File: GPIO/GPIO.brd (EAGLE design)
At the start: 35.6 x 29.8 mm, 30 parts

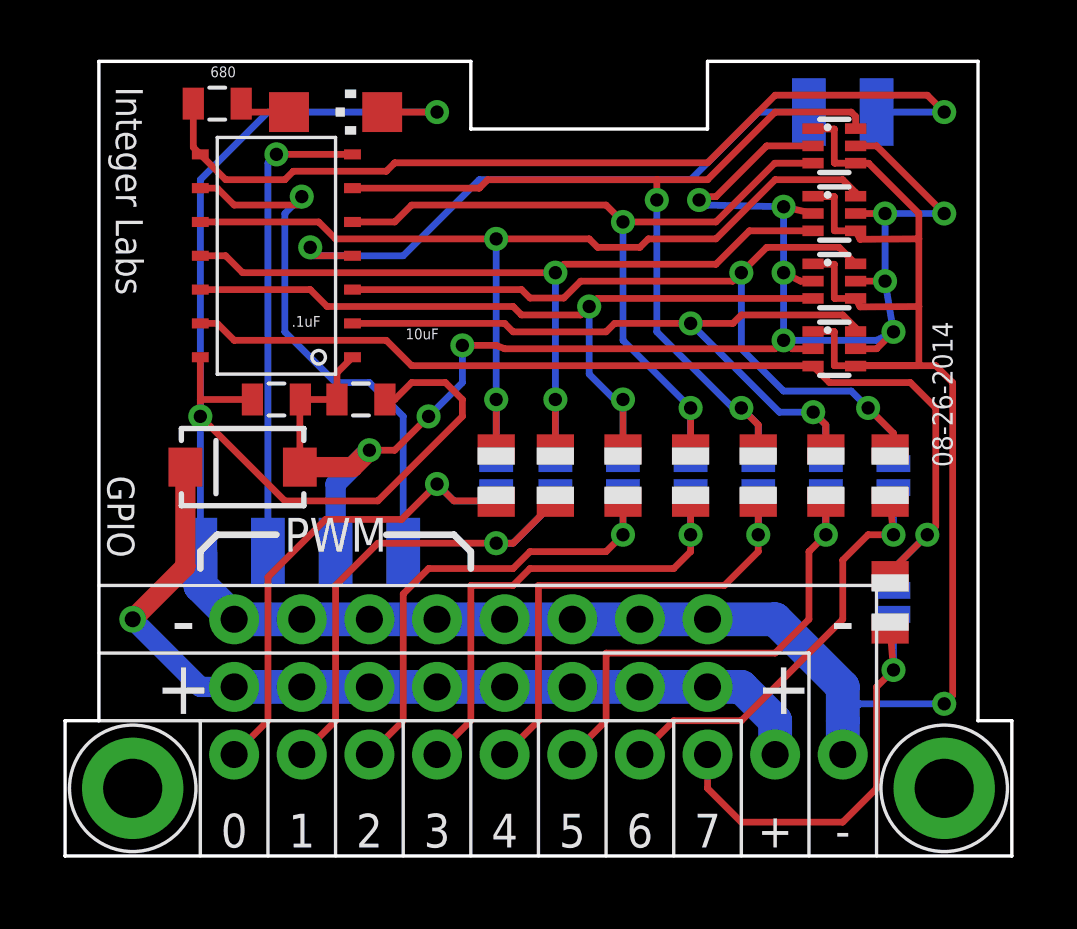
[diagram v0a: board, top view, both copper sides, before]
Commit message: Latest version of schematics and boards
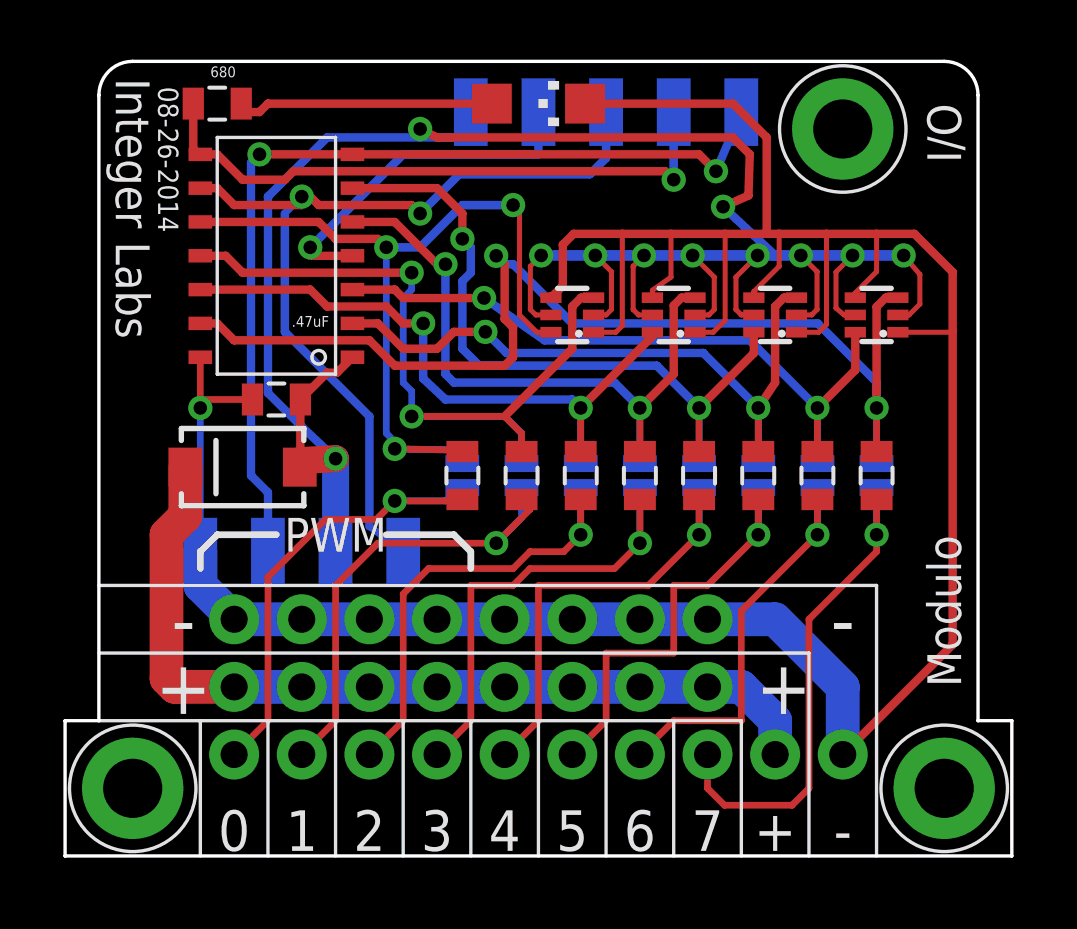
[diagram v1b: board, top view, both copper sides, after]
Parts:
- removed C1: 10uF, SparkFun-Capacitors:0805
- removed D0, D3, D5, D7: BAS70XY, diode:SOT363_PHILIPS
- added D26, D27, D28, D29: BAS70XY, diode:SOT363_PHILIPS
- C2: value .1uF -> .47uF
- R10, R11, R12, R13, R14, R15, R8, R9: value (none) -> 200; device adafruit:R0805 -> SparkFun-Resistors:0805
- moved LED 7.63 mm to (17.8, 28.3)
- moved R7 4.80 mm to (30.5, 14.3)
- moved R8 4.79 mm to (30.5, 14.3)
- moved R4 2.86 mm to (28.3, 14.3)
- moved R9 2.73 mm to (28.3, 14.3)
- moved R10 2.54 mm to (26.0, 14.3)
- moved R6 2.54 mm to (26.0, 14.3)
- moved R0 2.22 mm to (23.8, 14.3)
- moved R11 2.22 mm to (23.8, 14.3)
- moved R1 1.91 mm to (21.6, 14.3)
- moved R12 1.91 mm to (21.6, 14.3)
- moved R13 1.59 mm to (19.4, 14.3)
- moved R5 1.59 mm to (19.4, 14.3)
- moved R14 1.27 mm to (17.1, 14.3)
- moved R15 1.27 mm to (14.9, 14.3)
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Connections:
- net GND: now also D26.1, D26.4, D27.1, D27.4, D28.1, D28.4, D29.1, D29.4, U$4.BUS0; no longer C1.1, D0.1, D0.4, D3.1, D3.4, D5.1, D5.4, D7.1, D7.4, U$4.GND
- net GPIO0: now also D26.6; no longer D3.6
- net GPIO1: now also D26.3; no longer D3.3
- net GPIO2: now also D27.6; no longer D5.3
- net GPIO3: now also D27.3; no longer D0.3
- net GPIO4: now also D28.6; no longer D0.6
- net GPIO5: now also D28.3; no longer D7.6
- net GPIO6: now also D29.6; no longer D5.6
- net GPIO7: now also D29.3; no longer D7.3
- net MISO/LED: now also U$4.PROG3; no longer U$4.MISO
- net RESET: now also U$4.PROG1; no longer U$4.RESET
- net SCL/SCK: now also U$4.BUS3, U$4.PROG2; no longer U$4.SCL
- net SDA/MOSI: now also U$4.BUS1, U$4.PROG4; no longer U$4.SDA
- net VCC: now also D26.2, D26.5, D27.2, D27.5, D28.2, D28.5, D29.2, D29.5, U$4.BUS2, U$4.PROG0; no longer C1.2, D0.2, D0.5, D3.2, D3.5, D5.2, D5.5, D7.2, D7.5, U$4.VCC
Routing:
- net VCC: track 67.7 -> 87.3 mm
- net SDA/MOSI: track 17.9 -> 35.1 mm, vias 1 -> 2
- net SCL/SCK: track 20.6 -> 34.2 mm, vias 1 -> 2
- net GND: track 124.7 -> 112.0 mm, vias 3 -> 1
- net MISO/LED: track 34.5 -> 23.0 mm
- net RESET: track 23.2 -> 13.5 mm
- net N$5: track 1.93 -> 9.68 mm
- net GPIO4: track 34.8 -> 27.1 mm
- net GPIO2: track 32.1 -> 25.2 mm
- net GPIO6: track 33.0 -> 26.3 mm
- net GPIO3: track 30.4 -> 25.1 mm
- net GPIO0: track 36.7 -> 31.8 mm, vias 2 -> 3
- net GPIO7: track 38.5 -> 42.6 mm, vias 1 -> 2
- net GPIO5: track 29.3 -> 25.8 mm
- net P4: track 19.3 -> 16.8 mm
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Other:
- outline, holes or cut-outs redrawn
- board text added: "I/O"
- board text added: "Modulo"
- board text added: "resistor bypass"
- board text removed: "GPIO"

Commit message: Checkpointing PCB designs
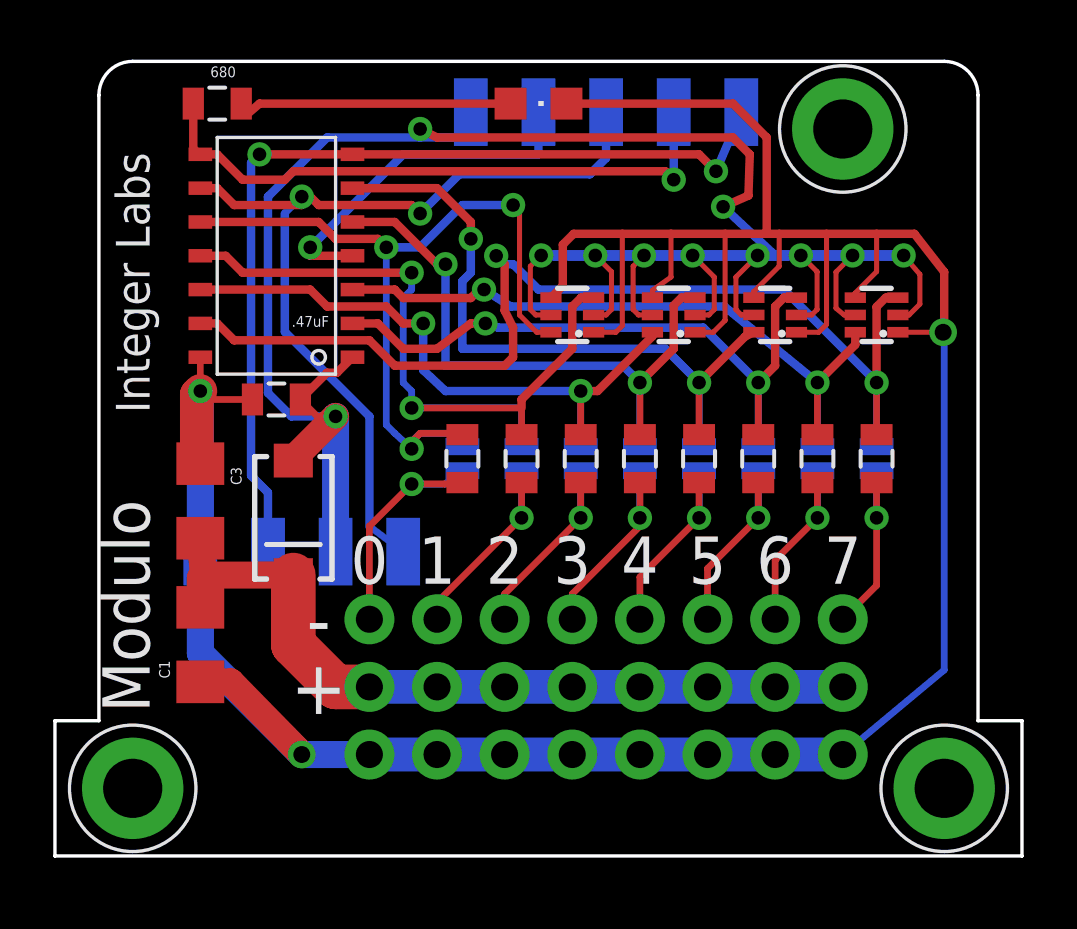
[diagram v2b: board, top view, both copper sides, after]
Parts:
- added C1, C3: (no value), SparkFun-Capacitors:1206
- JP2: device SparkFun-Connectors:1X10_NO_SILK -> SparkFun-Connectors:1X08_NO_SILK
- LED: device led:CHIPLED_1206 -> adafruit:CHIPLED_0805
- R10, R11, R12, R13, R14, R15, R8, R9: value 200 -> 130
- moved JP1 7.18 mm to (11.4, 3.81)
- moved JP2 7.18 mm to (11.4, 8.89)
- moved JP3 5.08 mm to (11.4, 6.35)
- moved D1 2.69 mm to (8.57, 12.7), turned to 270 degrees
- moved R0 0.63 mm to (23.8, 14.9)
- moved R1 0.63 mm to (21.6, 14.9)
- moved R10 0.63 mm to (26.0, 14.9)
- moved R11 0.63 mm to (23.8, 14.9)
- moved R12 0.63 mm to (21.6, 14.9)
- moved R13 0.63 mm to (19.4, 14.9)
- moved R14 0.63 mm to (17.1, 14.9)
- moved R15 0.63 mm to (14.9, 14.9)
- moved R2 0.63 mm to (14.9, 14.9)
- moved R3 0.63 mm to (17.1, 14.9)
- moved R4 0.63 mm to (28.3, 14.9)
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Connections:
- net GND: now also C1.1, C3.1; no longer JP2.10
- net VOUT: now also C1.2, C3.2; no longer JP2.9
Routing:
- net P7: track 19.8 -> 7.93 mm
- net P1: track 18.3 -> 8.22 mm
- net P3: track 17.6 -> 7.96 mm
- net P2: track 17.2 -> 8.09 mm
- net P4: track 16.8 -> 7.83 mm
- net P5: track 16.5 -> 7.69 mm
- net P0: track 18.4 -> 9.76 mm
- net GND: track 112.0 -> 120.6 mm, vias 1 -> 3
- net P6: track 15.6 -> 7.56 mm
- net VOUT: track 33.0 -> 29.9 mm
- net GPIO7: track 42.6 -> 41.0 mm
- net VCC: track 87.3 -> 88.3 mm
- net GPIO3: track 25.1 -> 24.2 mm
- net GPIO1: track 30.6 -> 29.8 mm
- net GPIO2: track 25.2 -> 24.5 mm
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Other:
- board size 35.6 x 29.8 mm -> 36.3 x 29.8 mm
- board text removed: "08-26-2014"
- board text removed: "I/O"
- board text removed: "Integer Labs"
- board text removed: "Modulo"
- board text removed: "PWM"
